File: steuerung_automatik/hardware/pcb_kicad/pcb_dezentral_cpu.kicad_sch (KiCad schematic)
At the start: 32 parts, among them J1 USB_C_Receptacle_USB2.0, SW2 SW_MEC_5E, U1 RP2040, U3 W25Q128JVS, U4 AMS1117-3.3, Y1 Crystal_GND24_Small

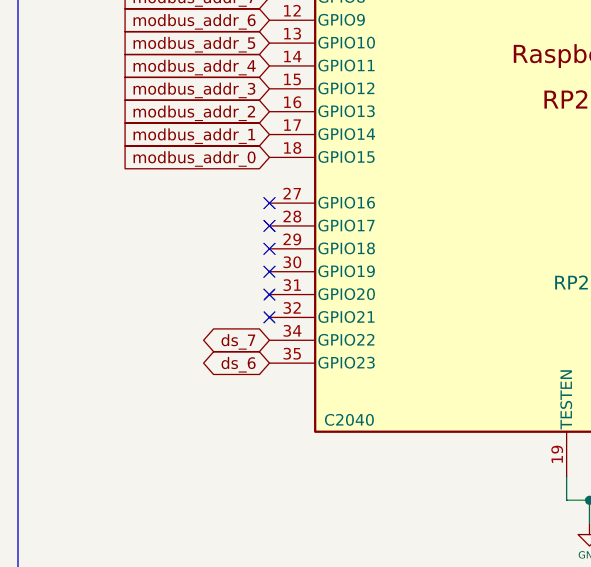
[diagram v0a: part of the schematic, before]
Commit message: Anpassungen von Peter
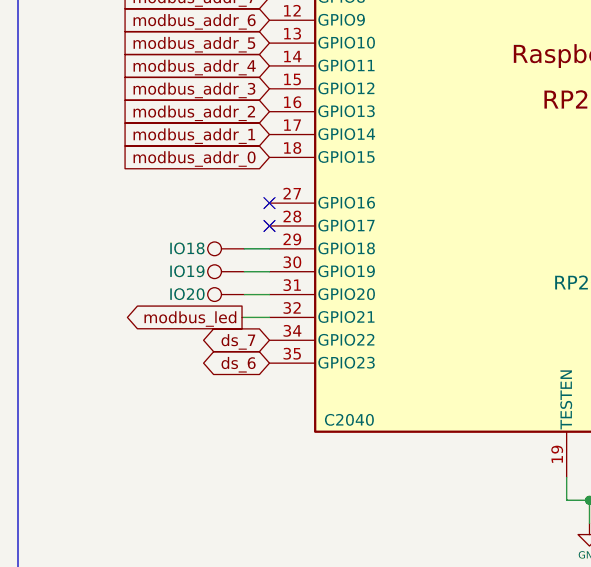
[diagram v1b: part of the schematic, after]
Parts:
- added IO18, IO19, IO20: TestPoint, TestPoint:TestPoint_Pad_D1.0mm, symbol Connector:TestPoint
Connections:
- net at U1.29 (GPIO18): now also IO18.1
- net at U1.30 (GPIO19): now also IO19.1
- net at U1.31 (GPIO20): now also IO20.1
- net modbus_led: now reaches U1.32 (GPIO21)
- no-connect marks 14 -> 10
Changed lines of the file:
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@@
   (junction (at 189.992 70.358) (diameter 0) (color 0 0 0 0)
   )
-  (no_connect (at 43.942 95.504))
   (no_connect (at 176.276 100.838))
   (no_connect (at 43.942 52.324))
   (no_connect (at 176.276 98.298))
   (no_connect (at 115.062 52.324))
-  (no_connect (at 43.942 92.964))
   (no_connect (at 43.942 90.424))
   (no_connect (at 43.942 87.884))
   (no_connect (at 115.062 54.864))
   (no_connect (at 43.942 54.864))
-  (no_connect (at 43.942 98.044))
-  (no_connect (at 43.942 100.584))
   (no_connect (at 43.942 59.944))
   (no_connect (at 43.942 57.404))
@@
     (stroke (width 0) (type solid))
   )
+  (wire (pts (xy 41.148 98.044) (xy 43.942 98.044))
+    (stroke (width 0) (type default))
+  )
   (wire (pts (xy 214.63 100.076) (xy 214.63 96.266))
     (stroke (width 0) (type default))
@@
     (stroke (width 0) (type solid))
   )
+  (wire (pts (xy 41.148 95.504) (xy 43.942 95.504))
+    (stroke (width 0) (type default))
+  )
   (wire (pts (xy 244.348 144.272) (xy 249.428 144.272))
     (stroke (width 0) (type solid))
@@
     (stroke (width 0) (type solid))
   )
+  (wire (pts (xy 41.148 92.964) (xy 43.942 92.964))
+    (stroke (width 0) (type default))
+  )
   (wire (pts (xy 187.706 77.978) (xy 187.706 79.248))
     (stroke (width 0) (type solid))
@@
   (wire (pts (xy 177.546 88.138) (xy 187.706 88.138))
     (stroke (width 0) (type solid))
+  )
+  (wire (pts (xy 40.894 100.584) (xy 43.942 100.584))
+    (stroke (width 0) (type default))
   )
   (wire (pts (xy 189.992 70.358) (xy 191.77 70.358))
@@
     )
   )
+  (global_label "modbus_led" (shape output) (at 40.894 100.584 180) (fields_autoplaced)
+    (effects (font (size 1.27 1.27)) (justify right))
+    (property "Intersheetrefs" "${INTERSHEET_REFS}" (at 26.6259 100.584 0)
+      (effects (font (size 1.27 1.27)) (justify right) hide)
+    )
+  )
   (global_label "modbus_addr_2" (shape input) (at 43.942 77.724 180) (fields_autoplaced)
     (effects (font (size 1.27 1.27)) (justify right))
@@
         (path "/35c47459-45a7-4753-acae-c8b47e7575e1/24d7d496-8920-4421-a637-0c9bf263a085"
           (reference "R907") (unit 1)
+        )
+      )
+    )
+  )
+  (symbol (lib_id "Connector:TestPoint") (at 41.148 95.504 90) (unit 1)
+    (in_bom yes) (on_board yes) (dnp no)
+    (property "Reference" "IO19" (at 34.798 95.504 90)
+      (effects (font (size 1.27 1.27)))
+    )
+    (property "Value" "TestPoint" (at 37.846 92.964 90)
+      (effects (font (size 1.27 1.27)) hide)
+    )
+    (property "Footprint" "TestPoint:TestPoint_Pad_D1.0mm" (at 41.148 90.424 0)
+      (effects (font (size 1.27 1.27)) hide)
+    )
+    (property "Datasheet" "~" (at 41.148 90.424 0)
+      (effects (font (size 1.27 1.27)) hide)
+    )
+    (pin "1")
+    (instances
+      (project "pcb_dezentral"
+        (path "/35c47459-45a7-4753-acae-c8b47e7575e1/24d7d496-8920-4421-a637-0c9bf263a085"
+          (reference "IO19") (unit 1)
         )
       )
@@
     )
   )
+  (symbol (lib_id "Connector:TestPoint") (at 41.148 92.964 90) (unit 1)
+    (in_bom yes) (on_board yes) (dnp no)
+    (property "Reference" "IO18" (at 34.798 92.964 90)
+      (effects (font (size 1.27 1.27)))
+    )
+    (property "Value" "TestPoint" (at 37.846 90.424 90)
+      (effects (font (size 1.27 1.27)) hide)
+    )
+    (property "Footprint" "TestPoint:TestPoint_Pad_D1.0mm" (at 41.148 87.884 0)
+      (effects (font (size 1.27 1.27)) hide)
+    )
+    (property "Datasheet" "~" (at 41.148 87.884 0)
+      (effects (font (size 1.27 1.27)) hide)
+    )
+    (pin "1")
+    (instances
+      (project "pcb_dezentral"
+        (path "/35c47459-45a7-4753-acae-c8b47e7575e1/24d7d496-8920-4421-a637-0c9bf263a085"
+          (reference "IO18") (unit 1)
+        )
+      )
+    )
+  )
   (symbol (lib_id "00_project_library:C") (at 199.136 36.322 0) (unit 1)
     (in_bom yes) (on_board yes) (dnp no)
@@
         )
       )
+    )
+  )
+  (symbol (lib_id "Connector:TestPoint") (at 41.148 98.044 90) (unit 1)
+    (in_bom yes) (on_board yes) (dnp no)
+    (property "Reference" "IO20" (at 34.798 98.044 90)
+      (effects (font (size 1.27 1.27)))
+    )
+    (property "Value" "TestPoint" (at 37.846 95.504 90)
+      (effects (font (size 1.27 1.27)) hide)
+    )
+    (property "Footprint" "TestPoint:TestPoint_Pad_D1.0mm" (at 41.148 92.964 0)
+      (effects (font (size 1.27 1.27)) hide)
+    )
+    (property "Datasheet" "~" (at 41.148 92.964 0)
+      (effects (font (size 1.27 1.27)) hide)
+    )
+    (pin "1")
+    (instances
+      (project "pcb_dezentral"
+        (path "/35c47459-45a7-4753-acae-c8b47e7575e1/24d7d496-8920-4421-a637-0c9bf263a085"
+          (reference "IO20") (unit 1)
+        )
+      )

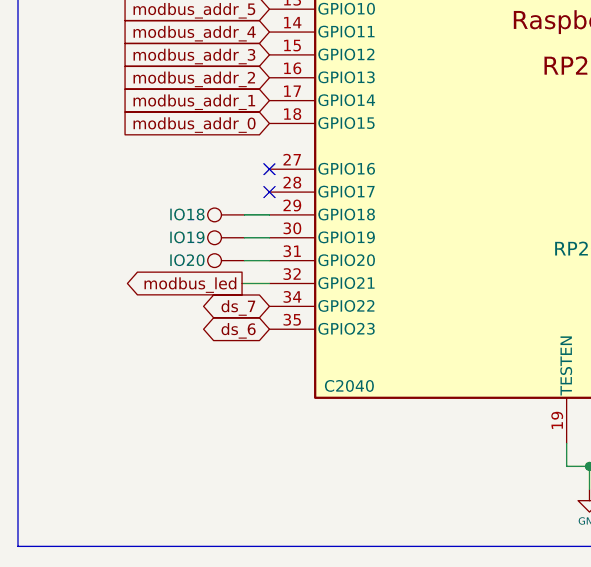
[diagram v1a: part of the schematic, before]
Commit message: pcb_dezentral v0.8
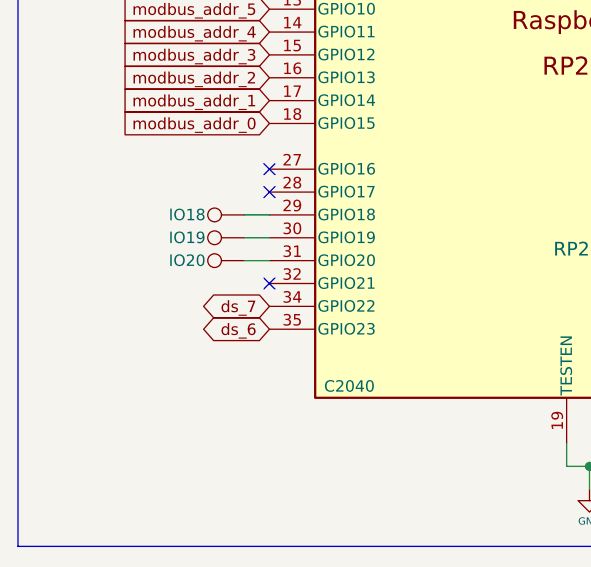
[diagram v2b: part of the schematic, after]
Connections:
- net modbus_led: no longer names the net of U1.32 (GPIO21)
- no-connect marks 10 -> 11
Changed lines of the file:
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@@
   (no_connect (at 176.276 98.298))
   (no_connect (at 115.062 52.324))
+  (no_connect (at 43.942 100.584))
   (no_connect (at 43.942 90.424))
   (no_connect (at 43.942 87.884))
@@
     (stroke (width 0) (type solid))
   )
-  (wire (pts (xy 40.894 100.584) (xy 43.942 100.584))
-    (stroke (width 0) (type default))
-  )
   (wire (pts (xy 189.992 70.358) (xy 191.77 70.358))
     (stroke (width 0) (type default))
@@
       (effects (font (size 1.27 1.27)) (justify right) hide)
     )
-  )
-  (global_label "modbus_led" (shape output) (at 40.894 100.584 180) (fields_autoplaced)
-    (effects (font (size 1.27 1.27)) (justify right))
-    (property "Intersheetrefs" "${INTERSHEET_REFS}" (at 26.6259 100.584 0)
-      (effects (font (size 1.27 1.27)) (justify right) hide)
-    )
